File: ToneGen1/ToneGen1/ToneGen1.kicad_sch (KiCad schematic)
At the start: 2 parts

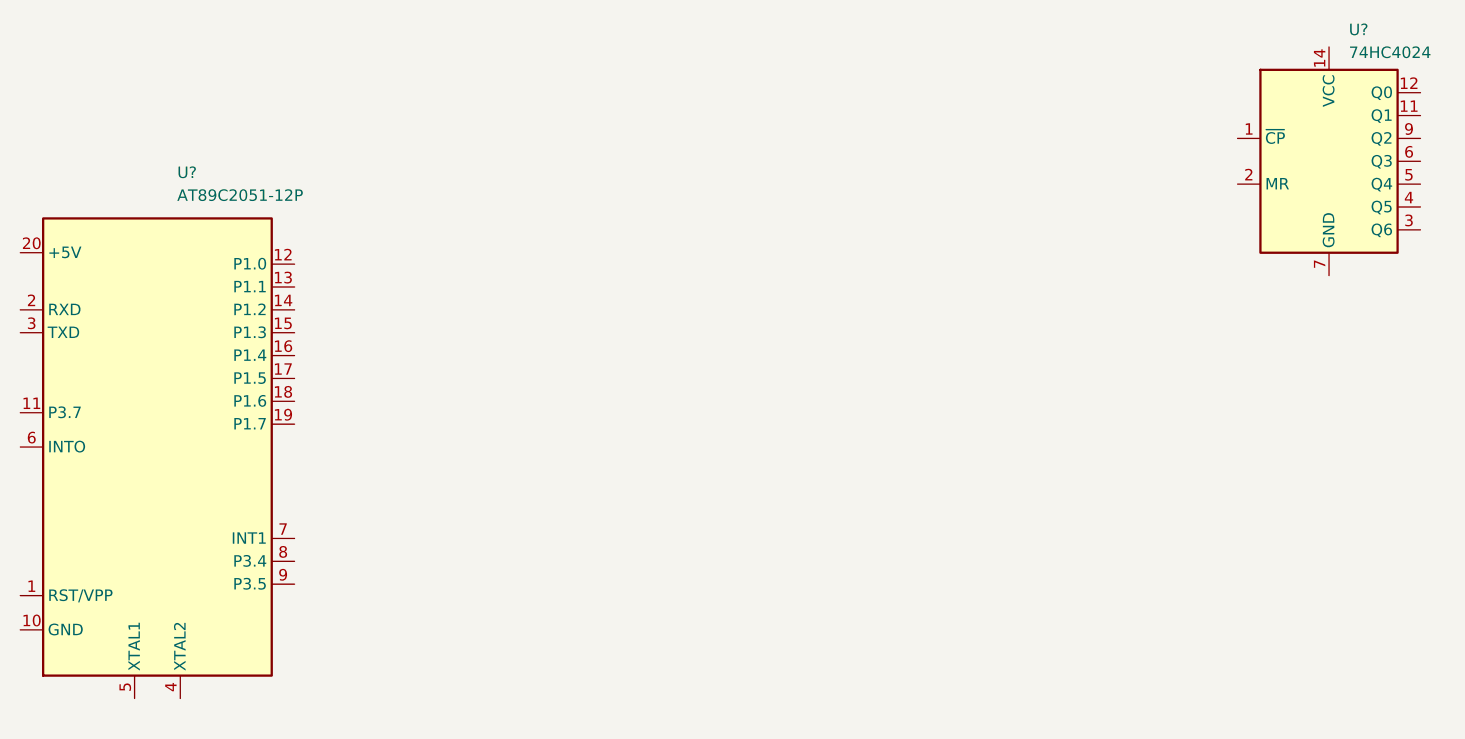
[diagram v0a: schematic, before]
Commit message: Add files via upload
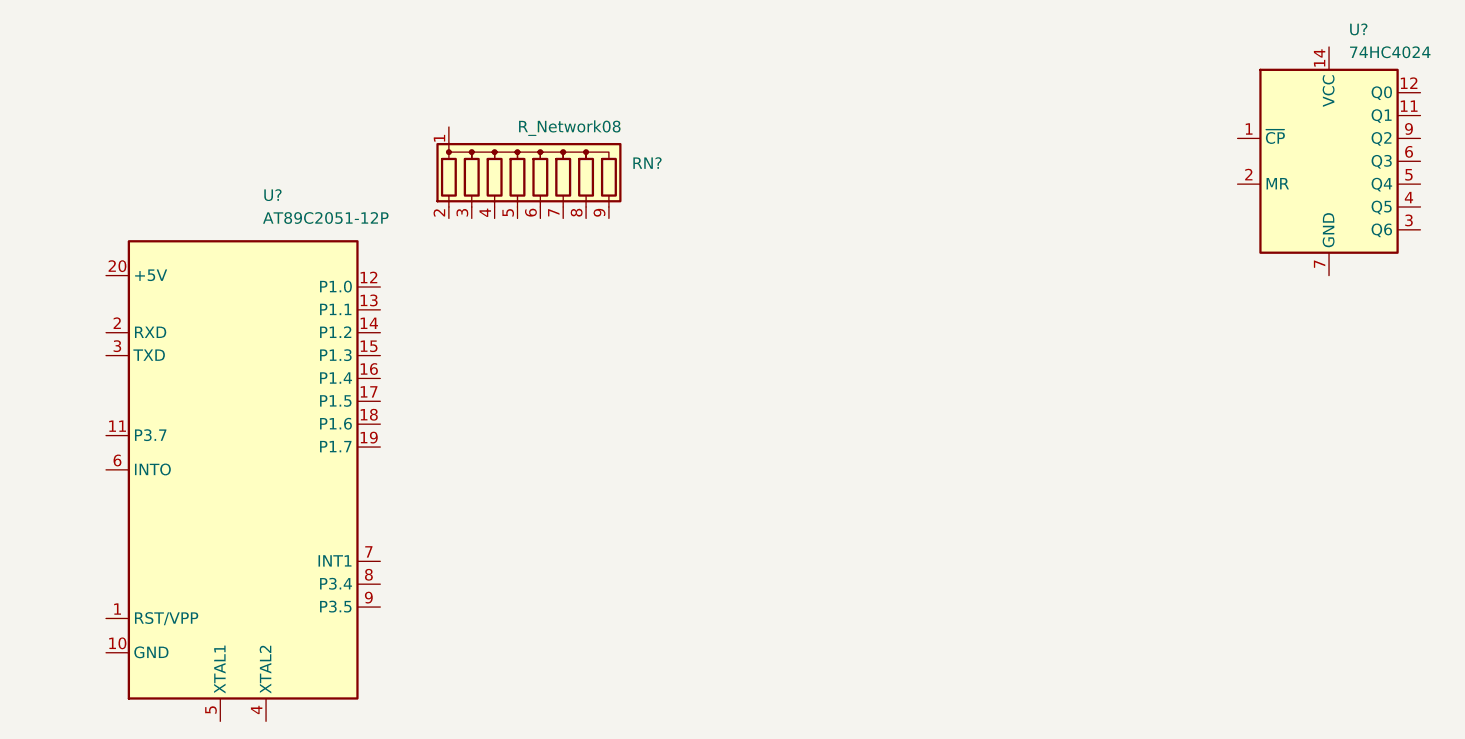
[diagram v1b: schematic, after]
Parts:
- added RN?: R_Network08, Resistor_THT:R_Array_SIP9, symbol Device:R_Network08
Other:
- moved on the sheet: U?
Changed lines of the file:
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@@
 	(paper "A4")
 	(symbol
+		(lib_id "Device:R_Network08")
+		(at 111.76 53.34 0)
+		(unit 1)
+		(exclude_from_sim no)
+		(in_bom yes)
+		(on_board yes)
+		(dnp no)
+		(property "Reference" "RN?"
+			(at 121.92 52.3239 0)
+			(effects
+				(font
+					(size 1.27 1.27)
+				)
+				(justify left)
+			)
+		)
+		(property "Value" "R_Network08"
+			(at 109.22 48.26 0)
+			(effects
+				(font
+					(size 1.27 1.27)
+				)
+				(justify left)
+			)
+		)
+		(property "Footprint" "Resistor_THT:R_Array_SIP9"
+			(at 123.825 53.34 90)
+			(effects
+				(font
+					(size 1.27 1.27)
+				)
+				(hide yes)
+			)
+		)
+		(property "Datasheet" "http://www.vishay.com/docs/31509/csc.pdf"
+			(at 111.76 53.34 0)
+			(effects
+				(font
+					(size 1.27 1.27)
+				)
+				(hide yes)
+			)
+		)
+		(property "Description" "8 resistor network, star topology, bussed resistors, small symbol"
+			(at 111.76 53.34 0)
+			(effects
+				(font
+					(size 1.27 1.27)
+				)
+				(hide yes)
+			)
+		)
+		(pin "7"
+		)
+		(pin "3"
+		)
+		(pin "8"
+		)
+		(pin "1"
+		)
+		(pin "9"
+		)
+		(pin "4"
+		)
+		(pin "6"
+		)
+		(pin "5"
+		)
+		(pin "2"
+		)
+		(instances
+			(project ""
+				(path "/5e9f077e-120e-43b0-a835-981431380f98"
+					(reference "RN?")
+					(unit 1)
+				)
+			)
+		)
+	)
+	(symbol
 		(lib_id "MCU_Microchip_8051:AT89C2051-12P")
-		(at 69.215 91.44 0)
+		(at 78.74 93.98 0)
 		(unit 1)
 		(exclude_from_sim no)
@@
 		(fields_autoplaced yes)
 		(property "Reference" "U?"
-			(at 71.4091 53.34 0)
+			(at 80.9341 55.88 0)
 			(effects
 				(font
@@
 		)
 		(property "Value" "AT89C2051-12P"
-			(at 71.4091 55.88 0)
+			(at 80.9341 58.42 0)
 			(effects
 				(font
@@
 		)
 		(property "Footprint" "Package_DIP:DIP-20_W7.62mm"
-			(at 12.319 130.556 0)
+			(at 21.844 133.096 0)
 			(effects
 				(font
@@
 		)
 		(property "Datasheet" "http://ww1.microchip.com/downloads/en/DeviceDoc/doc0368.pdf"
-			(at 17.907 133.096 0)
+			(at 27.432 135.636 0)
 			(effects
 				(font
@@
 		)
 		(property "Description" "12MHz, 2kB Flash, 128B SRAM, DIP-20"
-			(at 10.033 130.556 0)
+			(at 19.558 133.096 0)
 			(effects
 				(font
